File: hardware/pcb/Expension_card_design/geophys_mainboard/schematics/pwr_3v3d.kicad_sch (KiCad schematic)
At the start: 55 parts, among them Q1 AO3400A, Q2 AO3401A, Q3 AO3400A, U10 TPS54331DR, U18 TPS2116DRL, U19 TPS62933, U9 TPS2116DRL

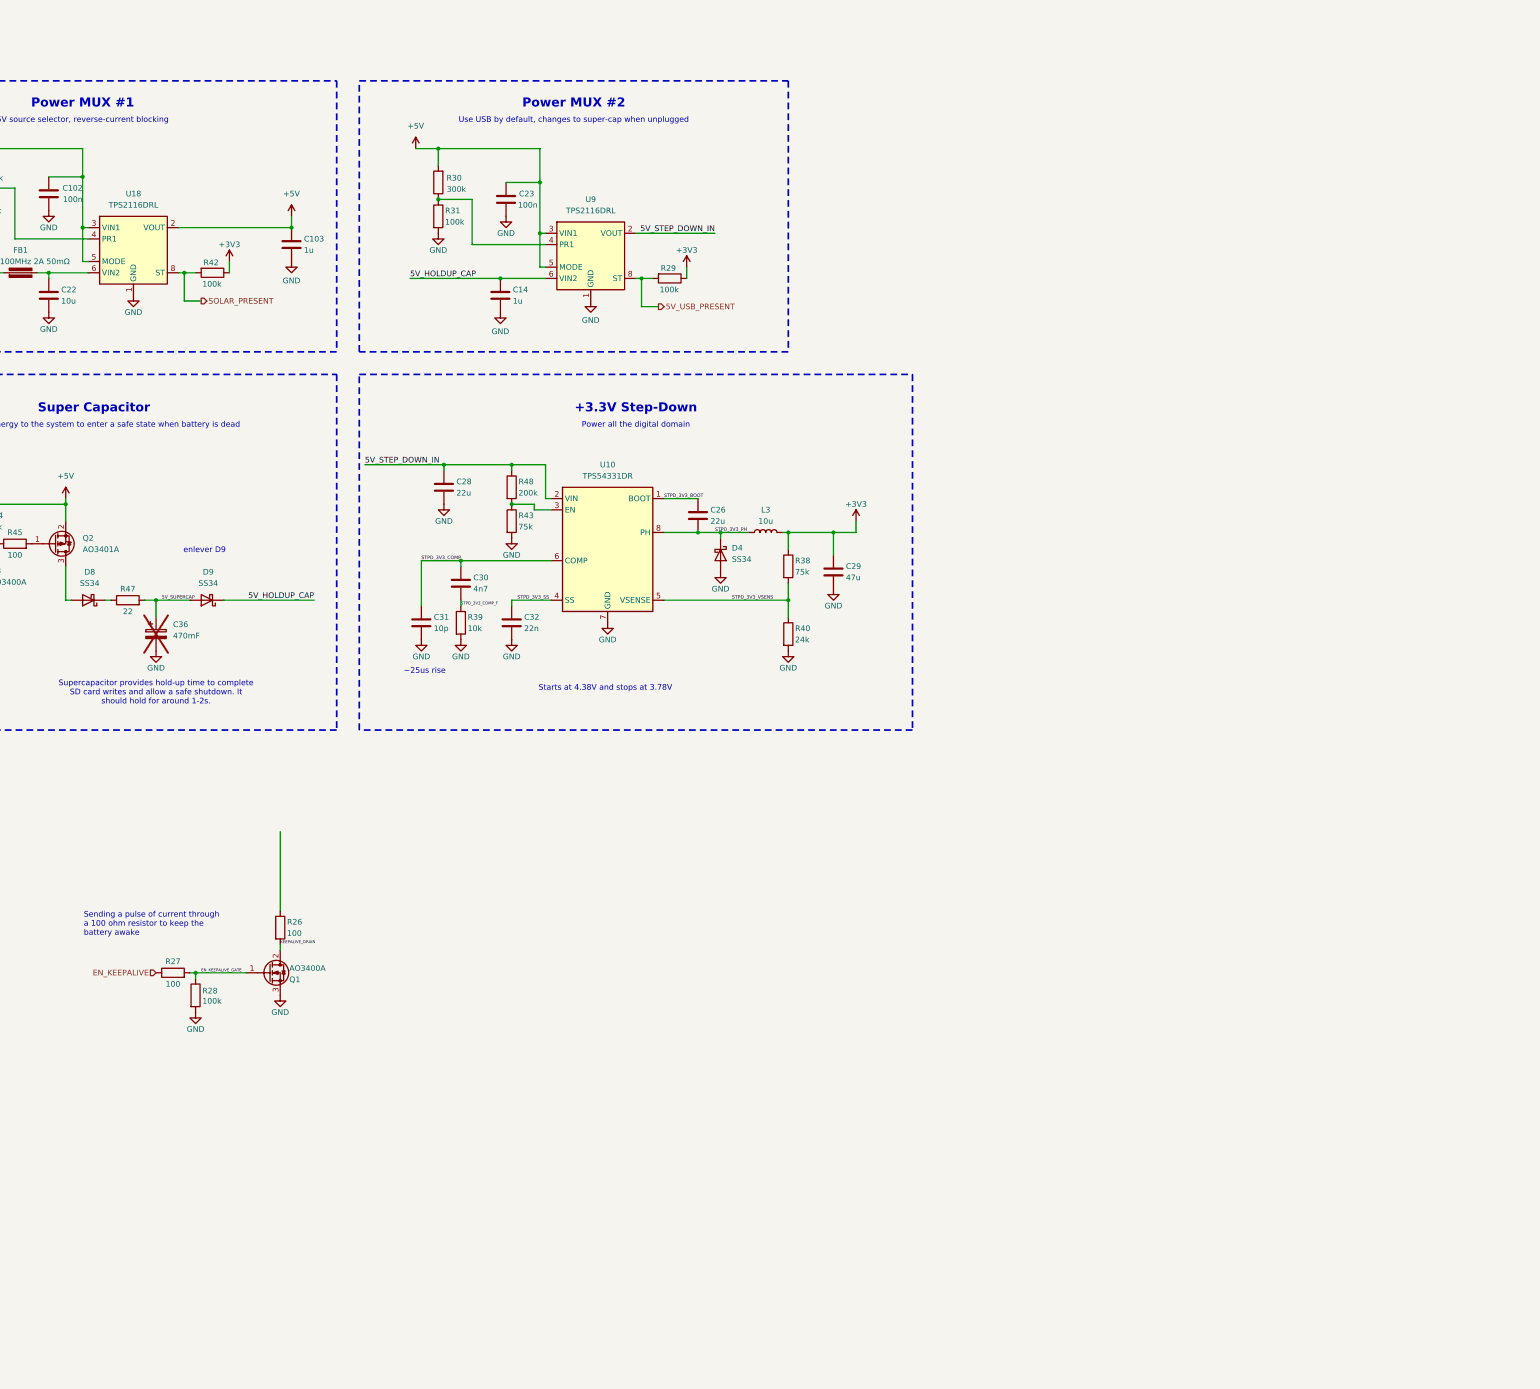
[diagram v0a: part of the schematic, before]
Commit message: Work in progress rev2
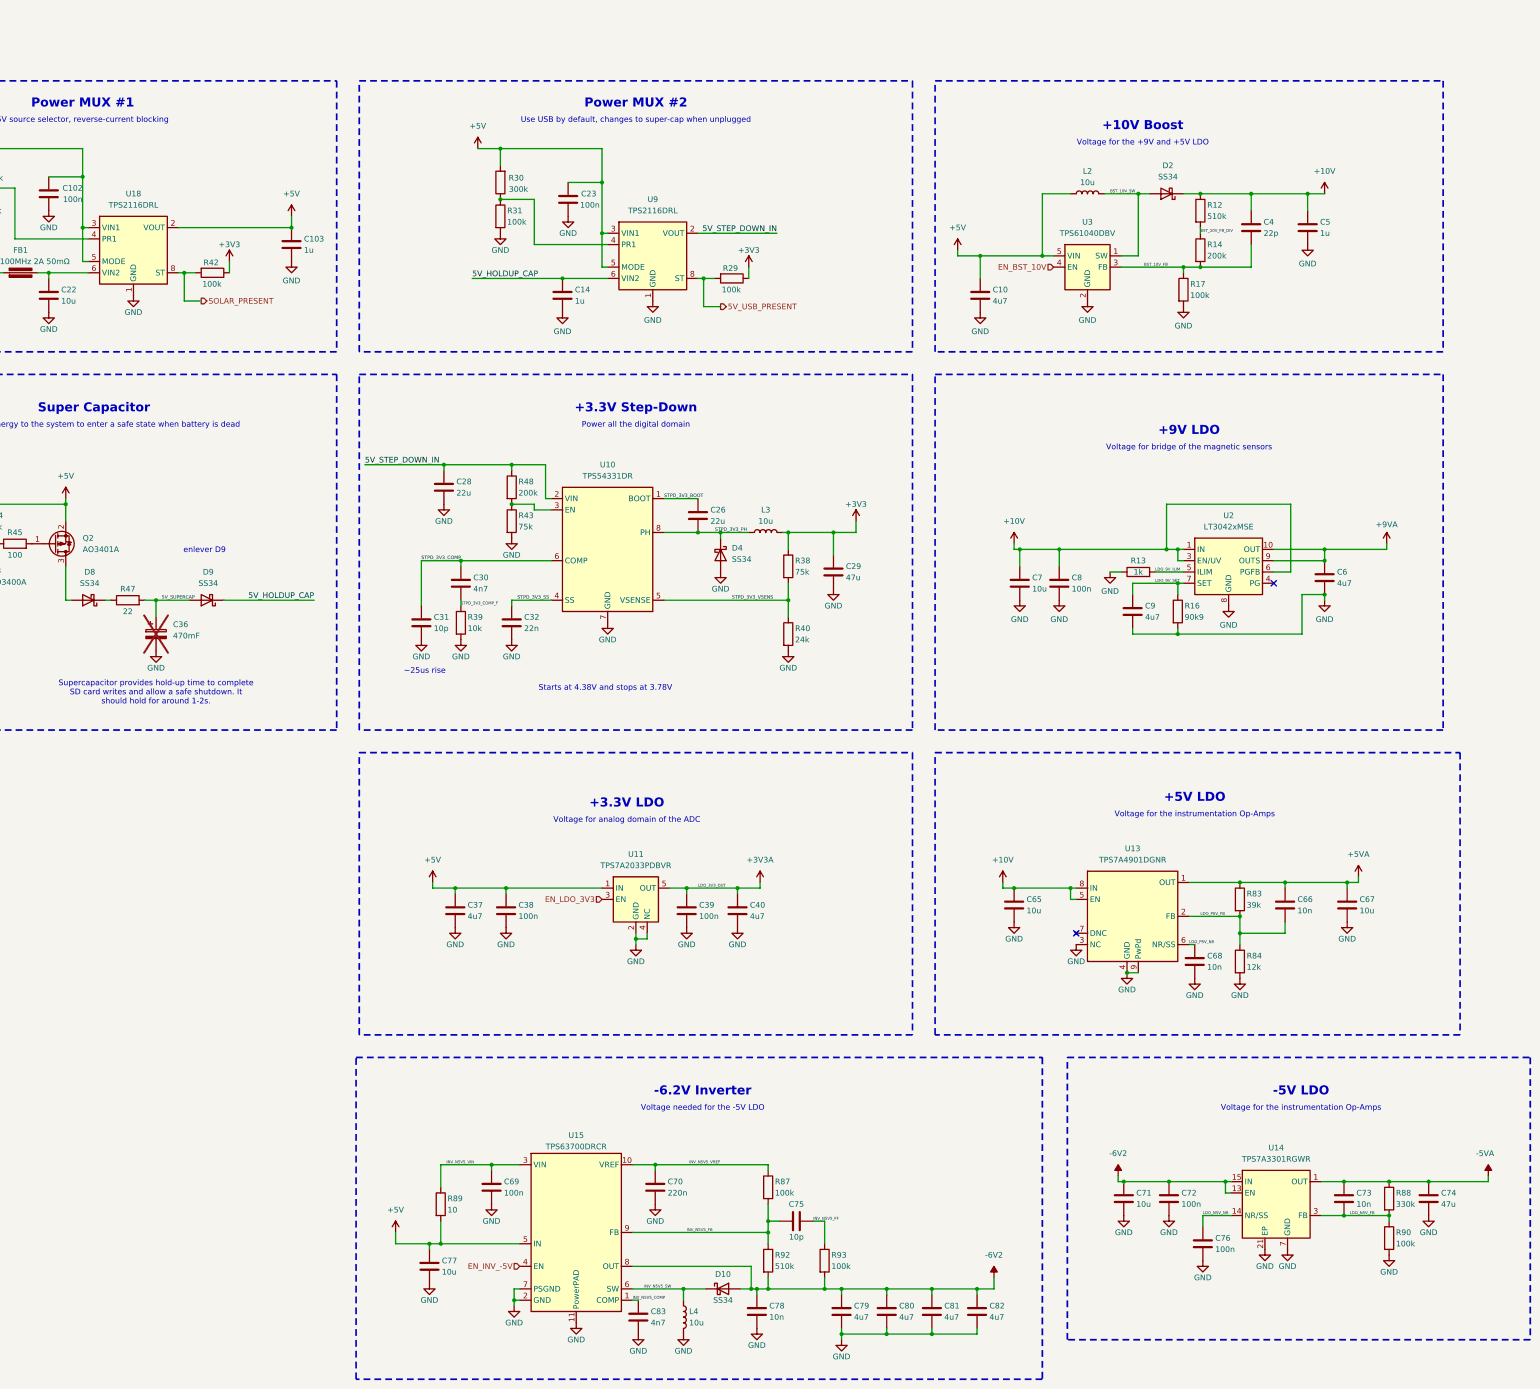
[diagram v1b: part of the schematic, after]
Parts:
- removed Q1: AO3400A, Package_TO_SOT_SMD:SOT-23, symbol magnode_symbols:AO3400A
- removed R26, R27: 100, Resistor_SMD:R_0603_1608Metric, symbol Device:R
- removed R28: 100k, Resistor_SMD:R_0603_1608Metric, symbol Device:R
- added C10, C37, C40, C6, C79, C80, C81, C82, C9: 4u7, Capacitor_SMD:C_1206_3216Metric, symbol Device:C
- added C38, C39, C69, C72, C76, C8: 100n, Capacitor_SMD:C_0603_1608Metric, symbol Device:C
- added C4: 22p, Capacitor_SMD:C_0603_1608Metric, symbol Device:C
- added C5: 1u, Capacitor_SMD:C_0805_2012Metric, symbol Device:C
- added C65, C67, C7, C71, C77: 10u, Capacitor_SMD:C_0805_2012Metric, symbol Device:C
- added C66, C68, C73, C78: 10n, Capacitor_SMD:C_0603_1608Metric, symbol Device:C
- added C70: 220n, Capacitor_SMD:C_0603_1608Metric, symbol Device:C
- added C74: 47u, Capacitor_SMD:C_1206_3216Metric, symbol Device:C
- added C75: 10p, Capacitor_SMD:C_0603_1608Metric, symbol Device:C
- added C83: 4n7, Capacitor_SMD:C_0603_1608Metric, symbol Device:C
- added D10, D2: SS34, Diode_SMD:D_SMA, symbol Device:D_Schottky
- added L2, L4: 10u, magnode_footprints:ZEMS0850-100M_8.5x8.0mm, symbol Device:L
- added R12, R92: 510k, Resistor_SMD:R_0603_1608Metric, symbol Device:R
- added R13: 1k, Resistor_SMD:R_0603_1608Metric, symbol Device:R
- added R14: 200k, Resistor_SMD:R_0603_1608Metric, symbol Device:R
- added R16: 90k9, Resistor_SMD:R_1206_3216Metric, symbol Device:R
- added R17, R87, R90, R93: 100k, Resistor_SMD:R_0603_1608Metric, symbol Device:R
- added R83: 39k, Resistor_SMD:R_0603_1608Metric, symbol Device:R
- added R84: 12k, Resistor_SMD:R_0603_1608Metric, symbol Device:R
- added R88: 330k, Resistor_SMD:R_0603_1608Metric, symbol Device:R
- added R89: 10, Resistor_SMD:R_0603_1608Metric, symbol Device:R
- added U11: TPS7A2033PDBVR, Package_TO_SOT_SMD:SOT-23-5, symbol magnode_symbols:TPS7A2033PDBVR
- added U13: TPS7A4901DGNR, magnode_footprints:HVSSOP-8-1EP_3x3mm_P0.65mm_EP1.57x1.89mm, symbol magnode_symbols:TPS7A4901
- added U14: TPS7A3301RGWR, Package_DFN_QFN:Texas_RGW0020A_VQFN-20-1EP_5x5mm_P0.65mm_EP3.15x3.15mm, symbol Regulator_Linear:TPS7A3301RGW
- added U15: TPS63700DRCR, Package_SON:VSON-10-1EP_3x3mm_P0.5mm_EP1.2x2mm, symbol magnode_symbols:TPS63700
- added U2: LT3042xMSE, Package_SO:MSOP-10-1EP_3x3mm_P0.5mm_EP1.68x1.88mm, symbol Regulator_Linear:LT3042xMSE
- added U3: TPS61040DBV, Package_TO_SOT_SMD:SOT-23-5, symbol Regulator_Switching:TPS61040DBV
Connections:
- net +5V: now also C10.1, C37.1, C38.1, C77.1, L2.1, R89.2, U11.1 (IN), U15.5 (IN), U3.5 (VIN)
- net GND: now also C10.2, C37.2, C38.2, C39.2, C40.2, C5.2, C6.2, C65.2, C67.2, C68.2, C69.2, C7.2, C70.2, C71.2, C72.2, C74.2, C76.2, C77.2, C78.2, C79.2, C8.2, C80.2, C81.2, C82.2, C83.2, C9.2, L4.2, R13.1, R16.2, R17.2, R84.2, R90.2, U11.2 (GND), U11.4 (NC), U13.3 (NC), U13.4 (GND), U13.9 (PwPd), U14.21 (EP), U14.7 (GND), U15.11 (PowerPAD), U15.2 (GND), U15.7 (PSGND), U2.11 (GND), U2.8 (GND), U3.2 (GND)
- new net +10V: C4.1, C5.1, C65.1, C7.1, C8.1, D2.1 (K), R12.1, U13.5 (EN), U13.8 (IN), U2.1 (IN), U2.2 (IN), U2.3 (EN/UV), U2.6 (PGFB)
- new net +3V3A: C39.1, C40.1, U11.5 (OUT)
- new net +5VA: C66.1, C67.1, R83.1, U13.1 (OUT)
- new net +9VA: C6.1, U2.10 (OUT), U2.9 (OUTS)
- new net -5VA: C73.1, C74.1, R88.1, U14.1 (OUT), U14.20 (OUT)
- new net -6V2: C71.1, C72.1, C78.1, C79.1, C80.1, C81.1, C82.1, D10.2 (A), R92.2, R93.2, U14.13 (EN), U14.15 (IN), U14.16 (IN), U15.8 (OUT)
- new net BST_10V_FB: C4.2, R14.2, R17.1, U3.3 (FB)
- new net BST_10V_FB_DIV: R12.2, R14.1
- new net BST_10V_SW: D2.2 (A), L2.2, U3.1 (SW)
- new net EN_BST_10V: U3.4 (EN)
- new net EN_INV_-5V: U15.4 (EN)
- new net EN_LDO_3V3: U11.3 (EN)
- new net INV_N5V5_COMP: C83.1, U15.1 (COMP)
- new net INV_N5V5_FB: C75.1, R87.2, R92.1, U15.9 (FB)
- new net INV_N5V5_FF: C75.2, R93.1
- new net INV_N5V5_SW: D10.1 (K), L4.1, U15.6 (SW)
- new net INV_N5V5_VIN: C69.1, R89.1, U15.3 (VIN)
- new net INV_N5V5_VREF: C70.1, R87.1, U15.10 (VREF)
- new net LDO_9V_ILIM: R13.2, U2.5 (ILIM)
- new net LDO_9V_SET: C9.1, R16.1, U2.7 (SET)
- new net LDO_N5V_FB: C73.2, R88.2, R90.1, U14.3 (FB)
- new net LDO_N5V_NR: C76.1, U14.14 (NR/SS)
- new net LDO_P5V_FB: C66.2, R83.2, R84.1, U13.2 (FB)
- new net LDO_P5V_NR: C68.1, U13.6 (NR/SS)
- no-connect marks 0 -> 2
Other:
- note added: "+10V Boost"
- note added: "+3.3V LDO"
- note added: "+5V LDO"
- note added: "+9V LDO"
- note added: "-5V LDO"
- note added: "-6.2V Inverter"
- note added: "Voltage for analog domain of the ADC"
- note added: "Voltage for bridge of the magnetic sensors"
- note added: "Voltage for the +9V and +5V LDO"
- note added: "Voltage for the instrumentation Op-Amps"
- note added: "Voltage needed for the -5V LDO"
- note removed: "Sending a pulse of current through a 100 ohm resistor to keep the battery awake"
- moved on the sheet: C14, C23, R29, R30, R31, U9
